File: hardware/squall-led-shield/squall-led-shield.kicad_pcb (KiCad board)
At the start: 2 copper layers, 25.4 x 21 mm, 10 parts, among them J1 SQUALL_HEADER, Q1 Q_2NMOS

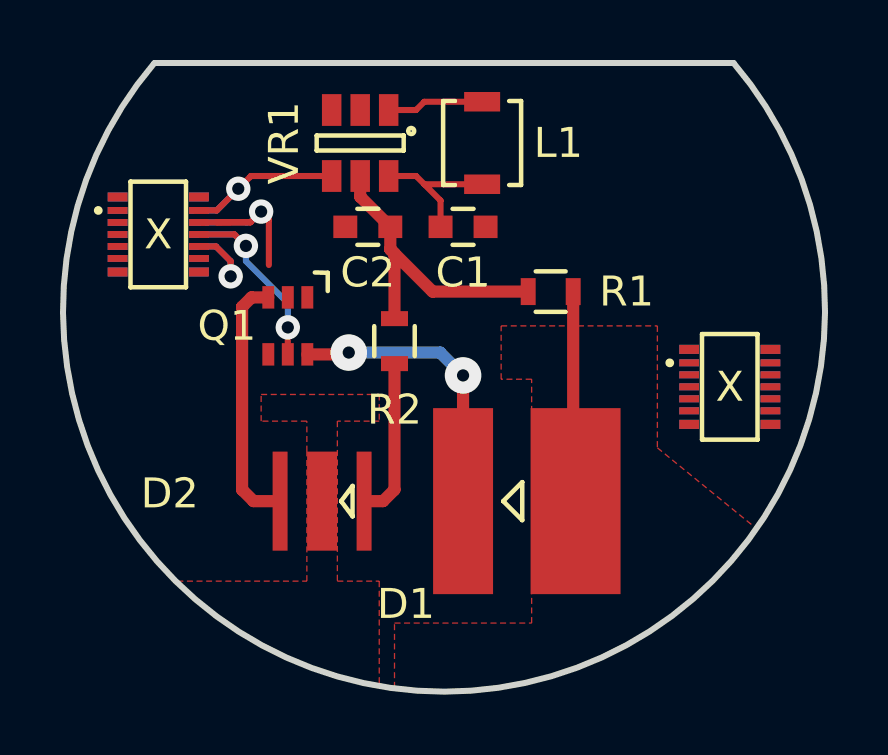
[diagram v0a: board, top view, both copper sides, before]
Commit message: WIP: Okay, the router is cool once you get it
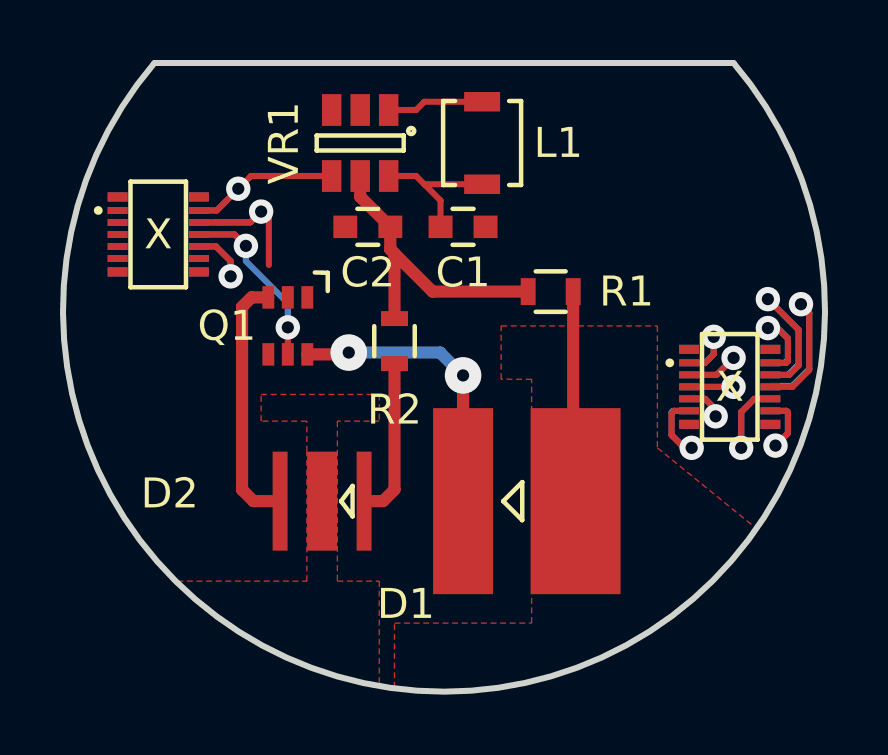
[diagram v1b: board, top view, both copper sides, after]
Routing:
- net Net-(J1-Pad16): track 0.00 -> 7.65 mm, vias 0 -> 1
- net Net-(J1-Pad14): track 0.00 -> 7.39 mm, vias 0 -> 1
- net Net-(J1-Pad18): track 0.00 -> 4.70 mm, vias 0 -> 1
- net Net-(J1-Pad19): track 0.00 -> 4.39 mm, vias 0 -> 1
- net Net-(J1-Pad12): track 0.00 -> 4.33 mm, vias 0 -> 1
- net Net-(J1-Pad20): track 0.00 -> 3.77 mm, vias 0 -> 1
- net Net-(J1-Pad13): track 0.00 -> 3.43 mm, vias 0 -> 1
- net Net-(J1-Pad11): track 0.00 -> 3.04 mm, vias 0 -> 1
- net Net-(J1-Pad15): track 0.00 -> 2.96 mm, vias 0 -> 1
- net Net-(J1-Pad17): track 0.00 -> 2.52 mm, vias 0 -> 1
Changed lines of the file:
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@@
     (thickness 1.6)
     (drawings 3)
-    (tracks 70)
+    (tracks 150)
     (zones 0)
     (modules 10)
@@
   (via (at 145.288 100.457) (size 0.8128) (drill 0.4064) (layers F.Cu B.Cu) (net 12))
   (segment (start 144.23 99.46) (end 144.799 99.46) (width 0.2032) (layer F.Cu) (net 12))
+  (segment (start 161.390368 102.472047) (end 161.390368 103.052832) (width 0.2032) (layer B.Cu) (net 13))
+  (segment (start 161.390368 103.052832) (end 161.1032 103.34) (width 0.2032) (layer B.Cu) (net 13))
+  (segment (start 161.1032 103.34) (end 160.57 103.34) (width 0.2032) (layer B.Cu) (net 13))
+  (segment (start 160.57 103.34) (end 161.1032 103.34) (width 0.2032) (layer F.Cu) (net 13))
+  (segment (start 161.1032 103.34) (end 161.390368 103.052832) (width 0.2032) (layer F.Cu) (net 13))
+  (segment (start 161.390368 103.052832) (end 161.390368 102.472047) (width 0.2032) (layer F.Cu) (net 13))
+  (via (at 161.390368 102.472047) (size 0.8128) (drill 0.4064) (layers F.Cu B.Cu) (net 13))
+  (segment (start 163.28 103.34) (end 163.767202 103.34) (width 0.2032) (layer B.Cu) (net 14))
+  (segment (start 163.522198 102.181198) (end 163.195 102.181198) (width 0.2032) (layer B.Cu) (net 14))
+  (segment (start 163.767202 103.34) (end 163.864001 103.243201) (width 0.2032) (layer B.Cu) (net 14))
+  (segment (start 163.864001 103.243201) (end 163.864001 102.523001) (width 0.2032) (layer B.Cu) (net 14))
+  (segment (start 163.864001 102.523001) (end 163.522198 102.181198) (width 0.2032) (layer B.Cu) (net 14))
+  (segment (start 163.28 103.34) (end 163.8132 103.34) (width 0.2032) (layer F.Cu) (net 14))
+  (segment (start 163.8132 103.34) (end 163.864001 103.289199) (width 0.2032) (layer F.Cu) (net 14))
+  (segment (start 163.864001 103.289199) (end 163.864001 102.536799) (width 0.2032) (layer F.Cu) (net 14))
+  (segment (start 163.864001 102.536799) (end 163.5084 102.181198) (width 0.2032) (layer F.Cu) (net 14))
+  (segment (start 163.5084 102.181198) (end 163.195 102.181198) (width 0.2032) (layer F.Cu) (net 14))
+  (via (at 163.195 102.181198) (size 0.8128) (drill 0.4064) (layers F.Cu B.Cu) (net 14))
+  (segment (start 162.052 103.174797) (end 161.486797 103.74) (width 0.2032) (layer F.Cu) (net 15))
+  (segment (start 161.486797 103.74) (end 160.57 103.74) (width 0.2032) (layer F.Cu) (net 15))
+  (segment (start 160.57 103.74) (end 161.486797 103.74) (width 0.2032) (layer B.Cu) (net 15))
+  (segment (start 161.486797 103.74) (end 162.052 103.174797) (width 0.2032) (layer B.Cu) (net 15))
+  (via (at 162.052 103.174797) (size 0.8128) (drill 0.4064) (layers F.Cu B.Cu) (net 15))
+  (segment (start 163.195 101.215995) (end 164.21961 102.240605) (width 0.2032) (layer F.Cu) (net 16))
+  (segment (start 164.21961 102.240605) (end 164.21961 103.436498) (width 0.2032) (layer F.Cu) (net 16))
+  (segment (start 164.21961 103.436498) (end 163.916108 103.74) (width 0.2032) (layer F.Cu) (net 16))
+  (segment (start 163.916108 103.74) (end 163.8132 103.74) (width 0.2032) (layer F.Cu) (net 16))
+  (segment (start 163.8132 103.74) (end 163.28 103.74) (width 0.2032) (layer F.Cu) (net 16))
+  (segment (start 163.28 103.74) (end 163.87011 103.74) (width 0.2032) (layer B.Cu) (net 16))
+  (segment (start 163.87011 103.74) (end 164.219611 103.390499) (width 0.2032) (layer B.Cu) (net 16))
+  (segment (start 164.219611 103.390499) (end 164.219611 102.240606) (width 0.2032) (layer B.Cu) (net 16))
+  (segment (start 164.219611 102.240606) (end 163.195 101.215995) (width 0.2032) (layer B.Cu) (net 16))
+  (via (at 163.195 101.215995) (size 0.8128) (drill 0.4064) (layers F.Cu B.Cu) (net 16))
+  (segment (start 162.052 104.14) (end 160.57 104.14) (width 0.2032) (layer B.Cu) (net 17))
+  (segment (start 160.57 104.14) (end 162.052 104.14) (width 0.2032) (layer F.Cu) (net 17))
+  (via (at 162.052 104.14) (size 0.8128) (drill 0.4064) (layers F.Cu B.Cu) (net 17))
+  (segment (start 164.298476 101.385524) (end 164.575221 101.662269) (width 0.2032) (layer B.Cu) (net 18))
+  (segment (start 164.575221 101.662269) (end 164.575221 103.537797) (width 0.2032) (layer B.Cu) (net 18))
+  (segment (start 164.575221 103.537797) (end 164.004017 104.109001) (width 0.2032) (layer B.Cu) (net 18))
+  (segment (start 164.004017 104.109001) (end 163.310999 104.109001) (width 0.2032) (layer B.Cu) (net 18))
+  (segment (start 163.310999 104.109001) (end 163.28 104.14) (width 0.2032) (layer B.Cu) (net 18))
+  (segment (start 163.28 104.14) (end 164.019016 104.14) (width 0.2032) (layer F.Cu) (net 18))
+  (segment (start 164.019016 104.14) (end 164.57522 103.583796) (width 0.2032) (layer F.Cu) (net 18))
+  (segment (start 164.57522 103.583796) (end 164.57522 101.662268) (width 0.2032) (layer F.Cu) (net 18))
+  (segment (start 164.57522 101.662268) (end 164.298476 101.385524) (width 0.2032) (layer F.Cu) (net 18))
+  (via (at 164.298476 101.385524) (size 0.8128) (drill 0.4064) (layers F.Cu B.Cu) (net 18))
+  (segment (start 161.454603 105.123367) (end 161.454603 104.891403) (width 0.2032) (layer B.Cu) (net 19))
+  (segment (start 161.454603 104.891403) (end 161.1032 104.54) (width 0.2032) (layer B.Cu) (net 19))
+  (segment (start 161.1032 104.54) (end 160.57 104.54) (width 0.2032) (layer B.Cu) (net 19))
+  (segment (start 160.57 104.54) (end 161.1032 104.54) (width 0.2032) (layer F.Cu) (net 19))
+  (segment (start 161.1032 104.54) (end 161.454603 104.891403) (width 0.2032) (layer F.Cu) (net 19))
+  (segment (start 161.454603 104.891403) (end 161.454603 105.123367) (width 0.2032) (layer F.Cu) (net 19))
+  (via (at 161.454603 105.123367) (size 0.8128) (drill 0.4064) (layers F.Cu B.Cu) (net 19))
+  (segment (start 162.306 106.172) (end 162.306 104.9808) (width 0.2032) (layer B.Cu) (net 20))
+  (segment (start 162.306 104.9808) (end 162.7468 104.54) (width 0.2032) (layer B.Cu) (net 20))
+  (segment (start 162.7468 104.54) (end 163.28 104.54) (width 0.2032) (layer B.Cu) (net 20))
+  (segment (start 163.28 104.54) (end 162.7468 104.54) (width 0.2032) (layer F.Cu) (net 20))
+  (segment (start 162.7468 104.54) (end 162.306 104.9808) (width 0.2032) (layer F.Cu) (net 20))
+  (segment (start 162.306 104.9808) (end 162.306 106.172) (width 0.2032) (layer F.Cu) (net 20))
+  (via (at 162.306 106.172) (size 0.8128) (drill 0.4064) (layers F.Cu B.Cu) (net 20))
+  (segment (start 160.57 104.94) (end 160.082798 104.94) (width 0.2032) (layer F.Cu) (net 21))
+  (segment (start 160.082798 104.94) (end 159.985999 105.036799) (width 0.2032) (layer F.Cu) (net 21))
+  (segment (start 159.985999 105.036799) (end 159.985999 105.756999) (width 0.2032) (layer F.Cu) (net 21))
+  (segment (start 159.985999 105.756999) (end 160.401 106.172) (width 0.2032) (layer F.Cu) (net 21))
+  (segment (start 160.401 106.172) (end 160.655 106.172) (width 0.2032) (layer F.Cu) (net 21))
+  (segment (start 160.57 104.94) (end 160.0368 104.94) (width 0.2032) (layer B.Cu) (net 21))
+  (segment (start 160.0368 104.94) (end 159.985999 104.990801) (width 0.2032) (layer B.Cu) (net 21))
+  (segment (start 159.985999 104.990801) (end 159.985999 105.743201) (width 0.2032) (layer B.Cu) (net 21))
+  (segment (start 159.985999 105.743201) (end 160.414798 106.172) (width 0.2032) (layer B.Cu) (net 21))
+  (segment (start 160.414798 106.172) (end 160.655 106.172) (width 0.2032) (layer B.Cu) (net 21))
+  (via (at 160.655 106.172) (size 0.8128) (drill 0.4064) (layers F.Cu B.Cu) (net 21))
+  (segment (start 163.449 106.098802) (end 163.864001 105.683801) (width 0.2032) (layer F.Cu) (net 22))
+  (segment (start 163.864001 105.683801) (end 163.864001 104.990801) (width 0.2032) (layer F.Cu) (net 22))
+  (segment (start 163.864001 104.990801) (end 163.8132 104.94) (width 0.2032) (layer F.Cu) (net 22))
+  (segment (start 163.8132 104.94) (end 163.28 104.94) (width 0.2032) (layer F.Cu) (net 22))
+  (segment (start 163.28 104.94) (end 163.8132 104.94) (width 0.2032) (layer B.Cu) (net 22))
+  (segment (start 163.8132 104.94) (end 163.864001 104.990801) (width 0.2032) (layer B.Cu) (net 22))
+  (segment (start 163.864001 104.990801) (end 163.864001 105.683801) (width 0.2032) (layer B.Cu) (net 22))
+  (segment (start 163.864001 105.683801) (end 163.449 106.098802) (width 0.2032) (layer B.Cu) (net 22))
+  (via (at 163.449 106.098802) (size 0.8128) (drill 0.4064) (layers F.Cu B.Cu) (net 22))
   (segment (start 151.468 94.912) (end 151.743 94.637) (width 0.2032) (layer F.Cu) (net 23))
   (segment (start 151.743 94.637) (end 153.67 94.637) (width 0.2032) (layer F.Cu) (net 23))
